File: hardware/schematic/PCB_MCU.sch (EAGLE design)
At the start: 136 parts, among them Q1 SS8050-G, Q2 SS8050-G, SW4 1825910-6, SW5 1825910-6, U14 MMSZ5225BT1G, U15 MMSZ5230BT1G

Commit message: Schematic updates
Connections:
- removed net 0: 19_PINOUT.19, 4PIN_I2C_TEST.4, C3.3OUT1.2, C3.3OUT10.2, C3.3OUT11.1, C3.3OUT12.1, C3.3OUT2.2, C3.3OUT3.1, C3.3OUT4.1, C3.3OUT5.2, C3.3OUT6.2, C3.3OUT7.1, C3.3OUT8.1, C3.3OUT9.2, CBUS.2, CENS.2, CENS1.2, CUSB.2, CUSB1.1, CUSB2.1, CUSB3.2, CUSB5.2, D14.K, D15.K, D16.K, D2.K, D3.K, D4.K, D6.K, D7.K, D8.K, I2C_USBC_IN.GND, I2C_USBC_IN.GND_2, RILIM.1, RILIM1.1, RILIM2.1, RU1.1, RU3.1, RUSB.2, RUSB1.2, RUSB2.2, RUSB3.2, RUSB6.2, RUSB7.2, SENSOR_PSWITCH.GND, SENSOR_USBA_IN.4, SERVO_PSWITCH.GND, STEPPER_P_SWITCH.GND, STEPPER_USBC_IN.GND, STEPPER_USBC_IN.GND_2, SW4.1, SW5.1, UART_USBC_IN.GND, UART_USBC_IN.GND_2, UART_USB_CONVERTER.GND
- net GND: now also 19_PINOUT.19, 4PIN_I2C_TEST.4, C3.3OUT1.2, C3.3OUT10.2, C3.3OUT11.1, C3.3OUT12.1, C3.3OUT2.2, C3.3OUT3.1, C3.3OUT4.1, C3.3OUT5.2, C3.3OUT6.2, C3.3OUT7.1, C3.3OUT8.1, C3.3OUT9.2, CBUS.2, CENS.2, CENS1.2, CUSB.2, CUSB1.1, CUSB2.1, CUSB3.2, CUSB5.2, D14.K, D15.K, D16.K, D2.K, D3.K, D4.K, D6.K, D7.K, D8.K, I2C_USBC_IN.GND, I2C_USBC_IN.GND_2, RILIM.1, RILIM1.1, RILIM2.1, RU1.1, RU3.1, RUSB.2, RUSB1.2, RUSB2.2, RUSB3.2, RUSB6.2, RUSB7.2, SENSOR_PSWITCH.GND, SENSOR_USBA_IN.4, SERVO_PSWITCH.GND, STEPPER_P_SWITCH.GND, STEPPER_USBC_IN.GND, STEPPER_USBC_IN.GND_2, SW4.1, SW5.1, UART_USBC_IN.GND, UART_USBC_IN.GND_2, UART_USB_CONVERTER.GND

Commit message: Schematic Updates
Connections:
- net N$60 renamed 3.3USBA
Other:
- note added: "Connector and Pinout"
- note added: "MCU"
- note added: "Power Swtiches"
- note added: "Regulators"
- note added: "SD Connector"
- note added: "UART-USB Converter"
- moved on the sheet: 19_PINOUT, 3.3V_REGULATOR, 4PIN_I2C_TEST, 5V_REGULATOR, BAT_JP, C3.3MCU, C3.3MCU1, C3.3OUT1, C3.3OUT10, C3.3OUT11, C3.3OUT12, C3.3OUT2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

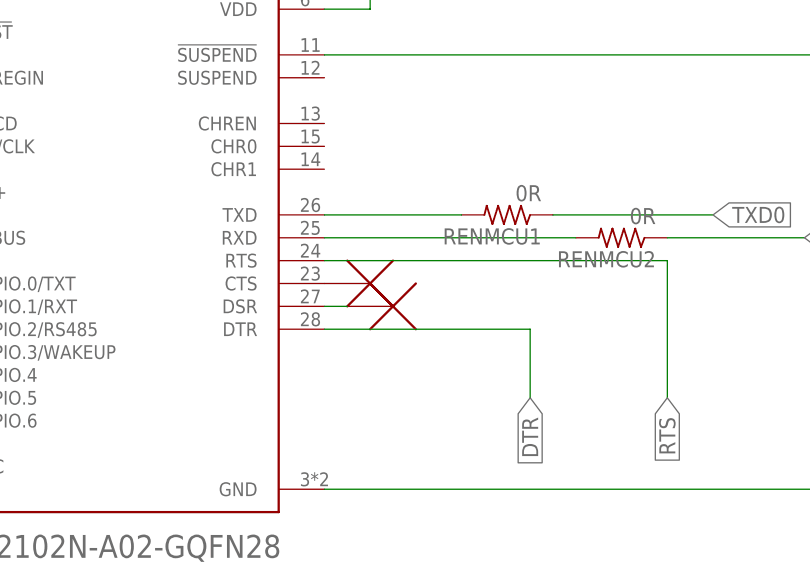
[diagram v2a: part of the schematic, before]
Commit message: Update PCB_MCU.sch
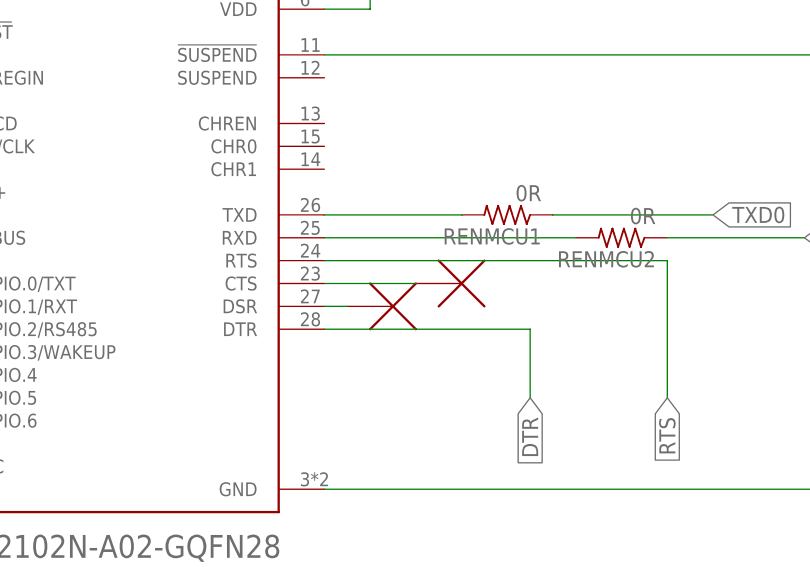
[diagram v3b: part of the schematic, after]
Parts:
- removed U$7: NC_MARKER, NC_MARKER:NC_MARKER
- added CTS_NC: NC_MARKER, NC_MARKER:NC_MARKER
- renumbered U$6 to DCD_NC
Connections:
- net N$1 renamed BOOT_3VREG
- net N$10 renamed TXD_UART_CONV
- net N$11 renamed BOOT_5VREG
- net N$12 renamed RXD_UART_CONV
- net N$13 renamed SW_5VREG
- net N$14 renamed VCC_5VREG
- net N$15 renamed PGOOD_5VREG
- net N$16 renamed MODE_5VREG
- net N$17 renamed TRIP_5VREG
- net N$18 renamed SS_REFIN_5VREG
- net N$19 renamed EN_5VREG
- net N$2 renamed SW_3VREG
- net N$22 renamed FB_5VREG
- net N$26 renamed SUSPEND
- net N$3 renamed VCC_3VREG
- net N$4 renamed PGOOD_3VREG
- net N$40 renamed RST_UART_CONV
- net N$41 renamed VBUS_UART_CONV
- net N$5 renamed EN_3VREG
- net N$51 renamed LED3_RLED9
- net N$52 renamed 3V3_MCU
- net N$53 renamed CC1_UART
- net N$54 renamed LED1_RSDCS
- net N$55 renamed LED_CONVERTER
- net N$56 renamed CC2_UART
- net N$57 renamed SD_CLK
- net N$58 renamed ILIM_SENSOR_S
- net N$59 renamed DATA_I_SD
- net N$6 renamed MODE_3VREG
- net N$61 renamed FAULT_SENSOR_S
- net N$62 renamed CC1_I2C
- net N$63 renamed CC2_I2C
- net N$66 renamed CC1_STEPPER
- net N$67 renamed ILIM_SERVO_S
- net N$68 renamed FAULT_SERVO_S
- net N$69 renamed CC2_STEPPER
- net N$7 renamed TRIP_3VREG
- net N$70 renamed ILIM_STEPPER_S
- net N$71 renamed FAULT_STEPPER_S
- net N$74 renamed 2+I_OP_AMP
- net N$75 renamed 2-I_OP_AMP
- net N$76 renamed 2O_OP_AMP
- net N$77 renamed 1I+_OP_AMP
- net N$78 renamed 1I-_OP_AMP
- net N$79 renamed 1O_OP_AMP
- net N$8 renamed SS_REFIN_3VREG
- net N$80 renamed LED2_RLED8
- net N$81 renamed DSR_NC
- net N$9 renamed FB_3VREG
- net N$91 renamed 5ASD
- net N$92 renamed 6ASD
- removed net N$86: U$7.P$1, UART_USB_CONVERTER.CTS
- new net CTS_NC: CTS_NC.P$1, UART_USB_CONVERTER.CTS
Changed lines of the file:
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@@
 <part name="X_3" library="ngspice-simulation" library_urn="urn:adsk.eagle:library:527439" deviceset="GND" device=""/>
 <part name="U$2" library="NC_MARKER" deviceset="NC_MARKER" device=""/>
-<part name="U$6" library="NC_MARKER" deviceset="NC_MARKER" device=""/>
-<part name="U$7" library="NC_MARKER" deviceset="NC_MARKER" device=""/>
+<part name="DCD_NC" library="NC_MARKER" deviceset="NC_MARKER" device=""/>
+<part name="CTS_NC" library="NC_MARKER" deviceset="NC_MARKER" device=""/>
 <part name="SENSOR_USBA_IN" library="USB-AP-S-RA-SMT" deviceset="USB-AP-S-RA-SMT" device=""/>
 <part name="SD_CONNECTOR" library="adafruit" library_urn="urn:adsk.eagle:library:420" deviceset="MICROSD" device="" package3d_urn="urn:adsk.eagle:package:6240723/1"/>
@@
 <instance part="X_3" gate="G$1" x="63.5" y="152.4" smashed="yes"/>
 <instance part="U$2" gate="G$1" x="-457.2" y="-147.32" smashed="yes" rot="R180"/>
-<instance part="U$6" gate="G$1" x="-515.62" y="-127" smashed="yes"/>
-<instance part="U$7" gate="G$1" x="-459.74" y="-144.78" smashed="yes" rot="R180"/>
+<instance part="DCD_NC" gate="G$1" x="-515.62" y="-127" smashed="yes"/>
+<instance part="CTS_NC" gate="G$1" x="-449.58" y="-144.78" smashed="yes" rot="R180"/>
 <instance part="SENSOR_USBA_IN" gate="A" x="7.62" y="198.12" smashed="yes" rot="R180">
 <attribute name="NAME" x="3.4544" y="192.8114" size="2.0828" layer="95" ratio="6" rot="SR180"/>
@@
 </busses>
 <nets>
-<net name="N$1" class="0">
+<net name="BOOT_3VREG" class="0">
 <segment>
 <pinref part="3.3V_REGULATOR" gate="A" pin="BOOT"/>
@@
 </segment>
 </net>
-<net name="N$2" class="0">
+<net name="SW_3VREG" class="0">
 <segment>
 <pinref part="3.3V_REGULATOR" gate="A" pin="SW"/>
@@
 </segment>
 </net>
-<net name="N$3" class="0">
+<net name="VCC_3VREG" class="0">
 <segment>
 <pinref part="3.3V_REGULATOR" gate="A" pin="VCC"/>
@@
 </segment>
 </net>
-<net name="N$4" class="0">
+<net name="PGOOD_3VREG" class="0">
 <segment>
 <pinref part="3.3V_REGULATOR" gate="A" pin="PGOOD"/>
@@
 </segment>
 </net>
-<net name="N$6" class="0">
+<net name="MODE_3VREG" class="0">
 <segment>
 <pinref part="3.3V_REGULATOR" gate="A" pin="MODE"/>
@@
 </segment>
 </net>
-<net name="N$7" class="0">
+<net name="TRIP_3VREG" class="0">
 <segment>
 <pinref part="3.3V_REGULATOR" gate="A" pin="TRIP"/>
@@
 </segment>
 </net>
-<net name="N$8" class="0">
+<net name="SS_REFIN_3VREG" class="0">
 <segment>
 <pinref part="3.3V_REGULATOR" gate="A" pin="SS_REFIN"/>
@@
 </segment>
 </net>
-<net name="N$5" class="0">
+<net name="EN_3VREG" class="0">
 <segment>
 <pinref part="RENB" gate="G$1" pin="2"/>
@@
 </segment>
 </net>
-<net name="N$9" class="0">
+<net name="FB_3VREG" class="0">
 <segment>
 <pinref part="RFBT" gate="G$1" pin="1"/>
@@
 </segment>
 </net>
-<net name="N$11" class="0">
+<net name="BOOT_5VREG" class="0">
 <segment>
 <pinref part="5V_REGULATOR" gate="A" pin="BOOT"/>
@@
 </segment>
 </net>
-<net name="N$13" class="0">
+<net name="SW_5VREG" class="0">
 <segment>
 <pinref part="5V_REGULATOR" gate="A" pin="SW"/>
@@
 </segment>
 </net>
-<net name="N$14" class="0">
+<net name="VCC_5VREG" class="0">
 <segment>
 <pinref part="5V_REGULATOR" gate="A" pin="VCC"/>
@@
 </segment>
 </net>
-<net name="N$15" class="0">
+<net name="PGOOD_5VREG" class="0">
 <segment>
 <pinref part="5V_REGULATOR" gate="A" pin="PGOOD"/>
@@
 </segment>
 </net>
-<net name="N$16" class="0">
+<net name="MODE_5VREG" class="0">
 <segment>
 <pinref part="5V_REGULATOR" gate="A" pin="MODE"/>
@@
 </segment>
 </net>
-<net name="N$17" class="0">
+<net name="TRIP_5VREG" class="0">
 <segment>
 <pinref part="5V_REGULATOR" gate="A" pin="TRIP"/>
@@
 </segment>
 </net>
-<net name="N$18" class="0">
+<net name="SS_REFIN_5VREG" class="0">
 <segment>
 <pinref part="5V_REGULATOR" gate="A" pin="SS_REFIN"/>
@@
 </segment>
 </net>
-<net name="N$19" class="0">
+<net name="EN_5VREG" class="0">
 <segment>
 <pinref part="RENB1" gate="G$1" pin="2"/>
@@
 </segment>
 </net>
-<net name="N$22" class="0">
+<net name="FB_5VREG" class="0">
 <segment>
 <pinref part="RFBT1" gate="G$1" pin="1"/>
@@
 </segment>
 </net>
-<net name="N$41" class="0">
+<net name="VBUS_UART_CONV" class="0">
 <segment>
 <pinref part="RU3" gate="G$1" pin="2"/>
@@
 </segment>
 </net>
-<net name="N$10" class="0">
+<net name="TXD_UART_CONV" class="0">
 <segment>
 <pinref part="UART_USB_CONVERTER" gate="G$1" pin="TXD"/>
@@
 </segment>
 </net>
-<net name="N$12" class="0">
+<net name="RXD_UART_CONV" class="0">
 <segment>
 <pinref part="UART_USB_CONVERTER" gate="G$1" pin="RXD"/>
@@
 </segment>
 </net>
-<net name="N$26" class="0">
+<net name="SUSPEND" class="0">
 <segment>
 <pinref part="UART_USB_CONVERTER" gate="G$1" pin="!SUSPEND"/>
@@
 </segment>
 </net>
-<net name="N$40" class="0">
+<net name="RST_UART_CONV" class="0">
 <segment>
 <pinref part="UART_USB_CONVERTER" gate="G$1" pin="!RST"/>
@@
 </segment>
 </net>
-<net name="N$52" class="0">
+<net name="3V3_MCU" class="0">
 <segment>
 <pinref part="RENMCU" gate="G$1" pin="2"/>
@@
 </segment>
 </net>
-<net name="N$53" class="0">
+<net name="CC1_UART" class="0">
 <segment>
 <pinref part="UART_USBC_IN" gate="A" pin="CC1"/>
@@
 </segment>
 </net>
-<net name="N$56" class="0">
+<net name="CC2_UART" class="0">
 <segment>
 <pinref part="UART_USBC_IN" gate="A" pin="CC2"/>
@@
 </segment>
 </net>
-<net name="N$58" class="0">
+<net name="ILIM_SENSOR_S" class="0">
 <segment>
 <pinref part="SENSOR_PSWITCH" gate="G$1" pin="ILIM"/>
@@
 </segment>
 </net>
-<net name="N$61" class="0">
+<net name="FAULT_SENSOR_S" class="0">
 <segment>
 <pinref part="SENSOR_PSWITCH" gate="G$1" pin="!FAULT"/>
@@
 </segment>
 </net>
-<net name="N$62" class="0">
+<net name="CC1_I2C" class="0">
 <segment>
 <pinref part="I2C_USBC_IN" gate="A" pin="CC1"/>
@@
 </segment>
 </net>
-<net name="N$63" class="0">
+<net name="CC2_I2C" class="0">
 <segment>
 <pinref part="I2C_USBC_IN" gate="A" pin="CC2"/>
@@
 </segment>
 </net>
-<net name="N$67" class="0">
+<net name="ILIM_SERVO_S" class="0">
 <segment>
 <pinref part="SERVO_PSWITCH" gate="G$1" pin="ILIM"/>
@@
 </segment>
 </net>
-<net name="N$68" class="0">
+<net name="FAULT_SERVO_S" class="0">
 <segment>
 <pinref part="SERVO_PSWITCH" gate="G$1" pin="!FAULT"/>
@@
 </segment>
 </net>
-<net name="N$66" class="0">
+<net name="CC1_STEPPER" class="0">
 <segment>
 <pinref part="STEPPER_USBC_IN" gate="A" pin="CC1"/>
@@
 </segment>
 </net>
-<net name="N$69" class="0">
+<net name="CC2_STEPPER" class="0">
 <segment>
 <pinref part="STEPPER_USBC_IN" gate="A" pin="CC2"/>
@@
 </segment>
 </net>
-<net name="N$70" class="0">
+<net name="ILIM_STEPPER_S" class="0">
 <segment>
 <pinref part="STEPPER_P_SWITCH" gate="G$1" pin="ILIM"/>
@@
 </segment>
 </net>
-<net name="N$71" class="0">
+<net name="FAULT_STEPPER_S" class="0">
 <segment>
 <pinref part="STEPPER_P_SWITCH" gate="G$1" pin="!FAULT"/>
@@
 </segment>
 </net>
-<net name="N$74" class="0">
+<net name="2+I_OP_AMP" class="0">
 <segment>
 <pinref part="RLEDOUT2" gate="G$1" pin="1"/>
@@
 </segment>
 </net>
-<net name="N$75" class="0">
+<net name="2-I_OP_AMP" class="0">
 <segment>
 <pinref part="RLEDOUT3" gate="G$1" pin="1"/>
@@
 </segment>
 </net>
-<net name="N$76" class="0">
+<net name="2O_OP_AMP" class="0">
 <segment>
 <pinref part="OP_AMP_LEDS" gate="A" pin="2OUT"/>
@@
 </segment>
 </net>
-<net name="N$77" class="0">
+<net name="1I+_OP_AMP" class="0">
 <segment>
 <pinref part="RLEDOUT" gate="G$1" pin="1"/>
@@
 </segment>
 </net>
-<net name="N$78" class="0">
+<net name="1I-_OP_AMP" class="0">
 <segment>
 <pinref part="RLEDOUT1" gate="G$1" pin="1"/>
@@
 </segment>
 </net>
-<net name="N$79" class="0">
+<net name="1O_OP_AMP" class="0">
 <segment>
 <pinref part="OP_AMP_LEDS" gate="A" pin="1OUT"/>
@@
 </segment>
 </net>
-<net name="N$80" class="0">
+<net name="LED2_RLED8" class="0">
 <segment>
 <pinref part="LED2" gate="G$1" pin="C"/>
@@
 </segment>
 </net>
-<net name="N$81" class="0">
+<net name="DSR_NC" class="0">
 <segment>
 <pinref part="UART_USB_CONVERTER" gate="G$1" pin="DSR"/>
@@
 <segment>
 <pinref part="UART_USB_CONVERTER" gate="G$1" pin="DCD"/>
-<pinref part="U$6" gate="G$1" pin="P$1"/>
-</segment>
-</net>
-<net name="N$86" class="0">
+<pinref part="DCD_NC" gate="G$1" pin="P$1"/>
+</segment>
+</net>
+<net name="CTS_NC" class="0">
 <segment>
 <pinref part="UART_USB_CONVERTER" gate="G$1" pin="CTS"/>
-<pinref part="U$7" gate="G$1" pin="P$1"/>
-</segment>
-</net>
-<net name="N$51" class="0">
+<pinref part="CTS_NC" gate="G$1" pin="P$1"/>
+<wire x1="-454.66" y1="-144.78" x2="-464.82" y2="-144.78" width="0.1524" layer="91"/>
+</segment>
+</net>
+<net name="LED3_RLED9" class="0">
 <segment>
 <pinref part="RLEDOUT9" gate="G$1" pin="1"/>
@@
 </segment>
 </net>
-<net name="N$54" class="0">
+<net name="LED1_RSDCS" class="0">
 <segment>
 <pinref part="LED1" gate="G$1" pin="C"/>
@@
 </segment>
 </net>
-<net name="N$55" class="0">
+<net name="LED_CONVERTER" class="0">
 <segment>
 <pinref part="LED1" gate="G$1" pin="A"/>
@@
 </segment>
 </net>
-<net name="N$57" class="0">
+<net name="SD_CLK" class="0">
 <segment>
 <pinref part="SD_CONNECTOR" gate="G$1" pin="SCLK"/>
@@
 </segment>
 </net>
-<net name="N$59" class="0">
+<net name="DATA_I_SD" class="0">
 <segment>
 <pinref part="SD_CONNECTOR" gate="G$1" pin="DATA_IN"/>
@@
 </segment>
 </net>
-<net name="N$91" class="0">
+<net name="5ASD" class="0">
 <segment>
 <pinref part="U$10" gate="G$1" pin="P$1"/>
@@
 </segment>
 </net>
-<net name="N$92" class="0">
+<net name="6ASD" class="0">
 <segment>
 <pinref part="DA_CONVERTER_SD" gate="A" pin="6A"/>
